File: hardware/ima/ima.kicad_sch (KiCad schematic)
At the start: 8 parts, among them J1 DM3AT-SF-PEJM5, U1 STM32F722RETx, U2 PCM5102A, Y1 Crystal, Y2 830055951, Y3 Crystal_GND24

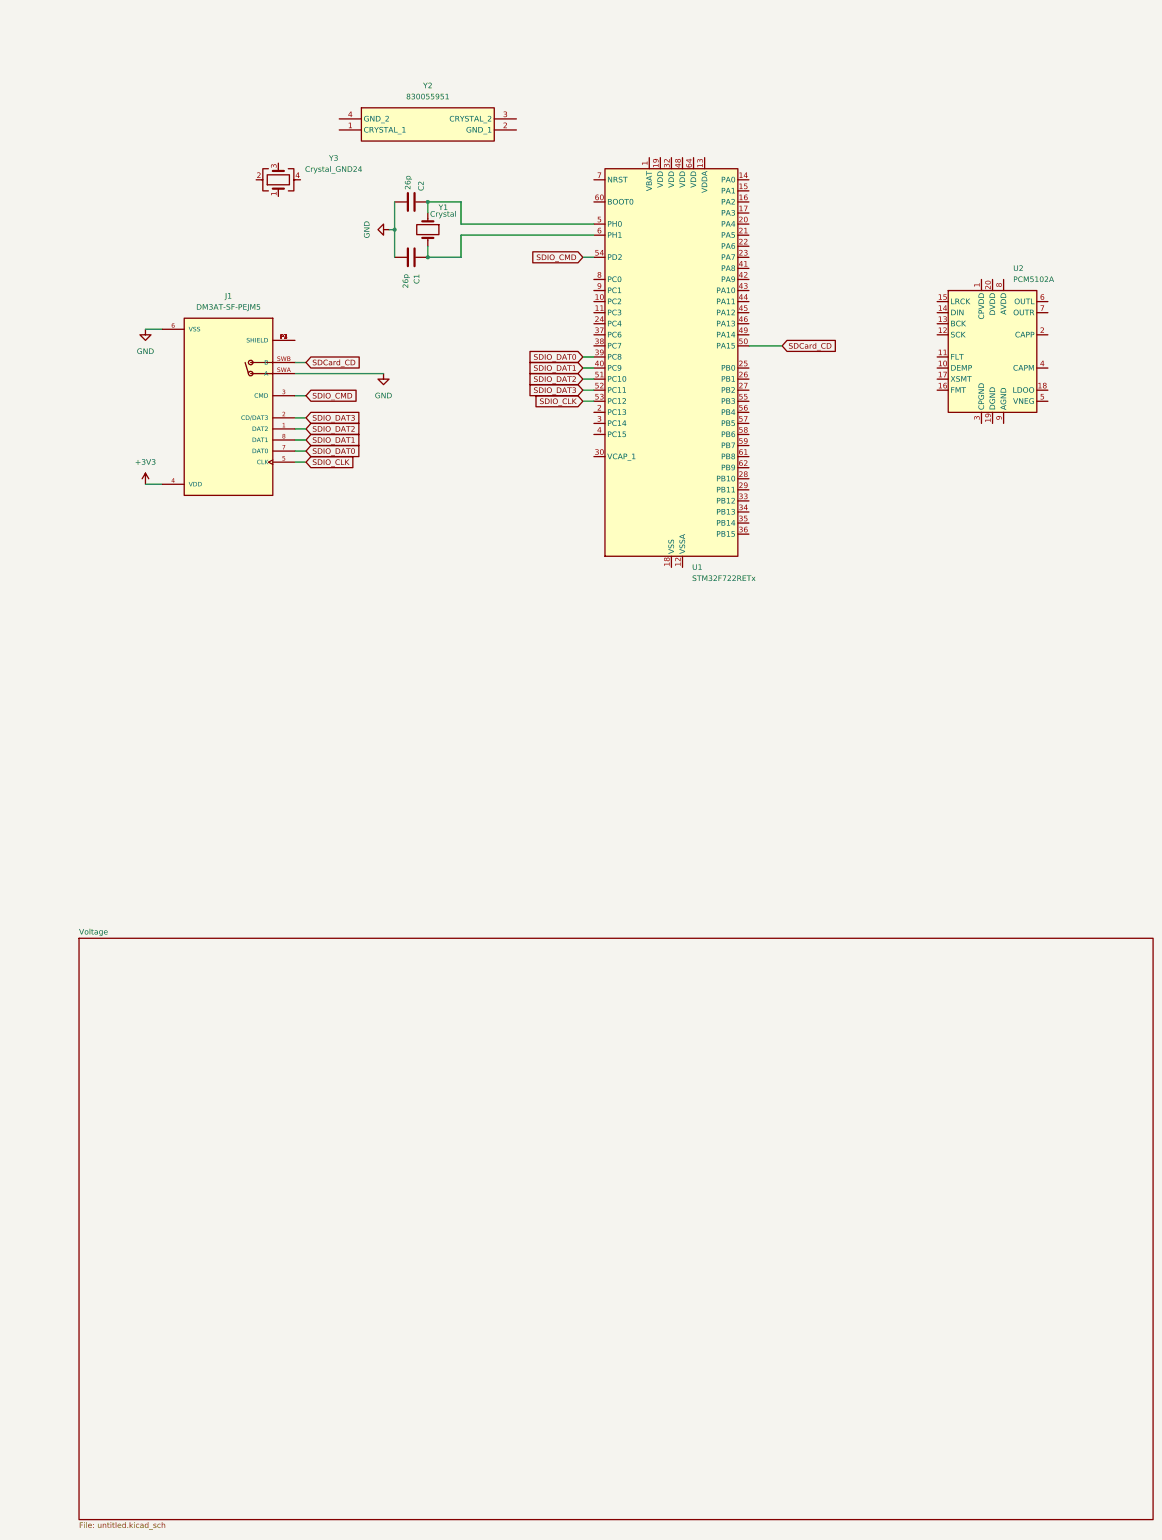
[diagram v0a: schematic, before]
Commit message: update docs
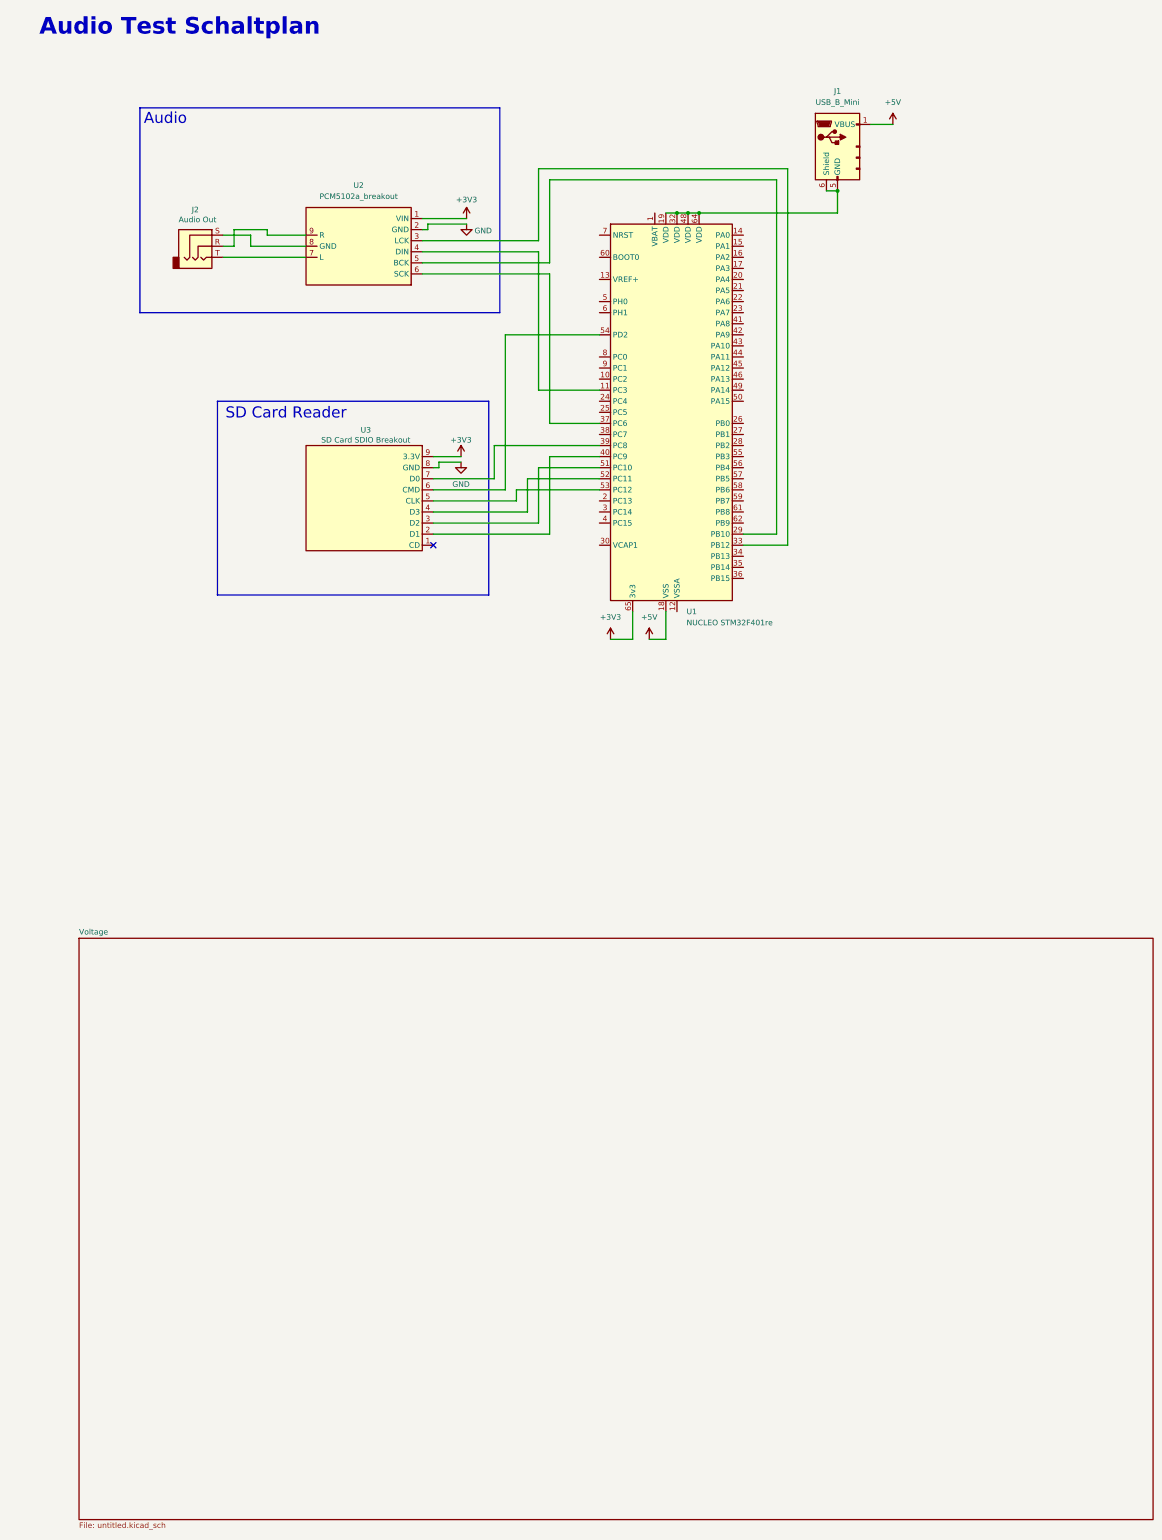
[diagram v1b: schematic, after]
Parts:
- removed C1, C2: 26p, symbol Device:C
- removed J1: DM3AT-SF-PEJM5, DM3AT-SF-PEJM5:HRS_DM3AT-SF-PEJM5, symbol SD Card Connector:DM3AT-SF-PEJM5
- removed U1: STM32F722RETx, Package_QFP:LQFP-64_10x10mm_P0.5mm, symbol MCU_ST_STM32F7:STM32F722RETx
- removed U2: PCM5102A, Package_SO:TSSOP-20_4.4x6.5mm_P0.65mm, symbol Audio:PCM5102A
- removed Y1: Crystal, symbol Device:Crystal
- removed Y2: 830055951, 830055951, symbol 16MHz Quartz:830055951
- removed Y3: Crystal_GND24, symbol Device:Crystal_GND24
- added J1: USB_B_Mini, symbol Connector:USB_B_Mini
- added J2: Audio Out, symbol Connector_Audio:AudioJack3
- added U1: NUCLEO STM32F401re, Package_QFP:LQFP-64_10x10mm_P0.5mm, symbol MCU_ST_STM32F4:STM32F401RETx
- added U2: PCM5102a_breakout, symbol New_Library:PCM5102a_breakout
- added U3: SD Card SDIO Breakout, symbol New_Library:Waveshare_SD_Card_Breakout
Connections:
- net +3V3: now also U1.65 (3v3), U2.1 (VIN), U3.9 (3.3V)
- net GND: now also U2.2 (GND), U3.8 (GND)
- new net: U1.11 (PC3), U2.4 (DIN)
- new net: J1.5 (GND), J1.6 (Shield), U1.19 (VDD), U1.32 (VDD), U1.48 (VDD), U1.64 (VDD)
- new net: U1.29 (PB10), U2.5 (BCK)
- new net: U1.33 (PB12), U2.3 (LCK)
- new net: U1.37 (PC6), U2.6 (SCK)
- new net: U1.39 (PC8), U3.7 (D0)
- new net: U1.40 (PC9), U3.2 (D1)
- new net: U1.51 (PC10), U3.3 (D2)
- new net: U1.52 (PC11), U3.4 (D3)
- new net: U1.53 (PC12), U3.5 (CLK)
- new net: U1.54 (PD2), U3.6 (CMD)
- new net: J2.R, U2.9 (R)
- new net: J2.S, U2.8 (GND)
- new net: J2.T, U2.7 (L)
- new net +5V: J1.1 (VBUS), U1.18 (VSS), U1.31 (VSS), U1.47 (VSS), U1.63 (VSS)
- no-connect marks 0 -> 1
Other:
- note added: "Audio"
- note added: "Audio Test Schaltplan"
- note added: "SD Card Reader"
